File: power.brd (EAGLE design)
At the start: 136 x 136 mm, 38 parts, among them CN1 21700, CN2 21700, CN3 21700, CN4 21700, CN5 15PIN 0.5MM, Q1 IRLML6244, Q2 IRLML6244, U1 MAX17320G20+

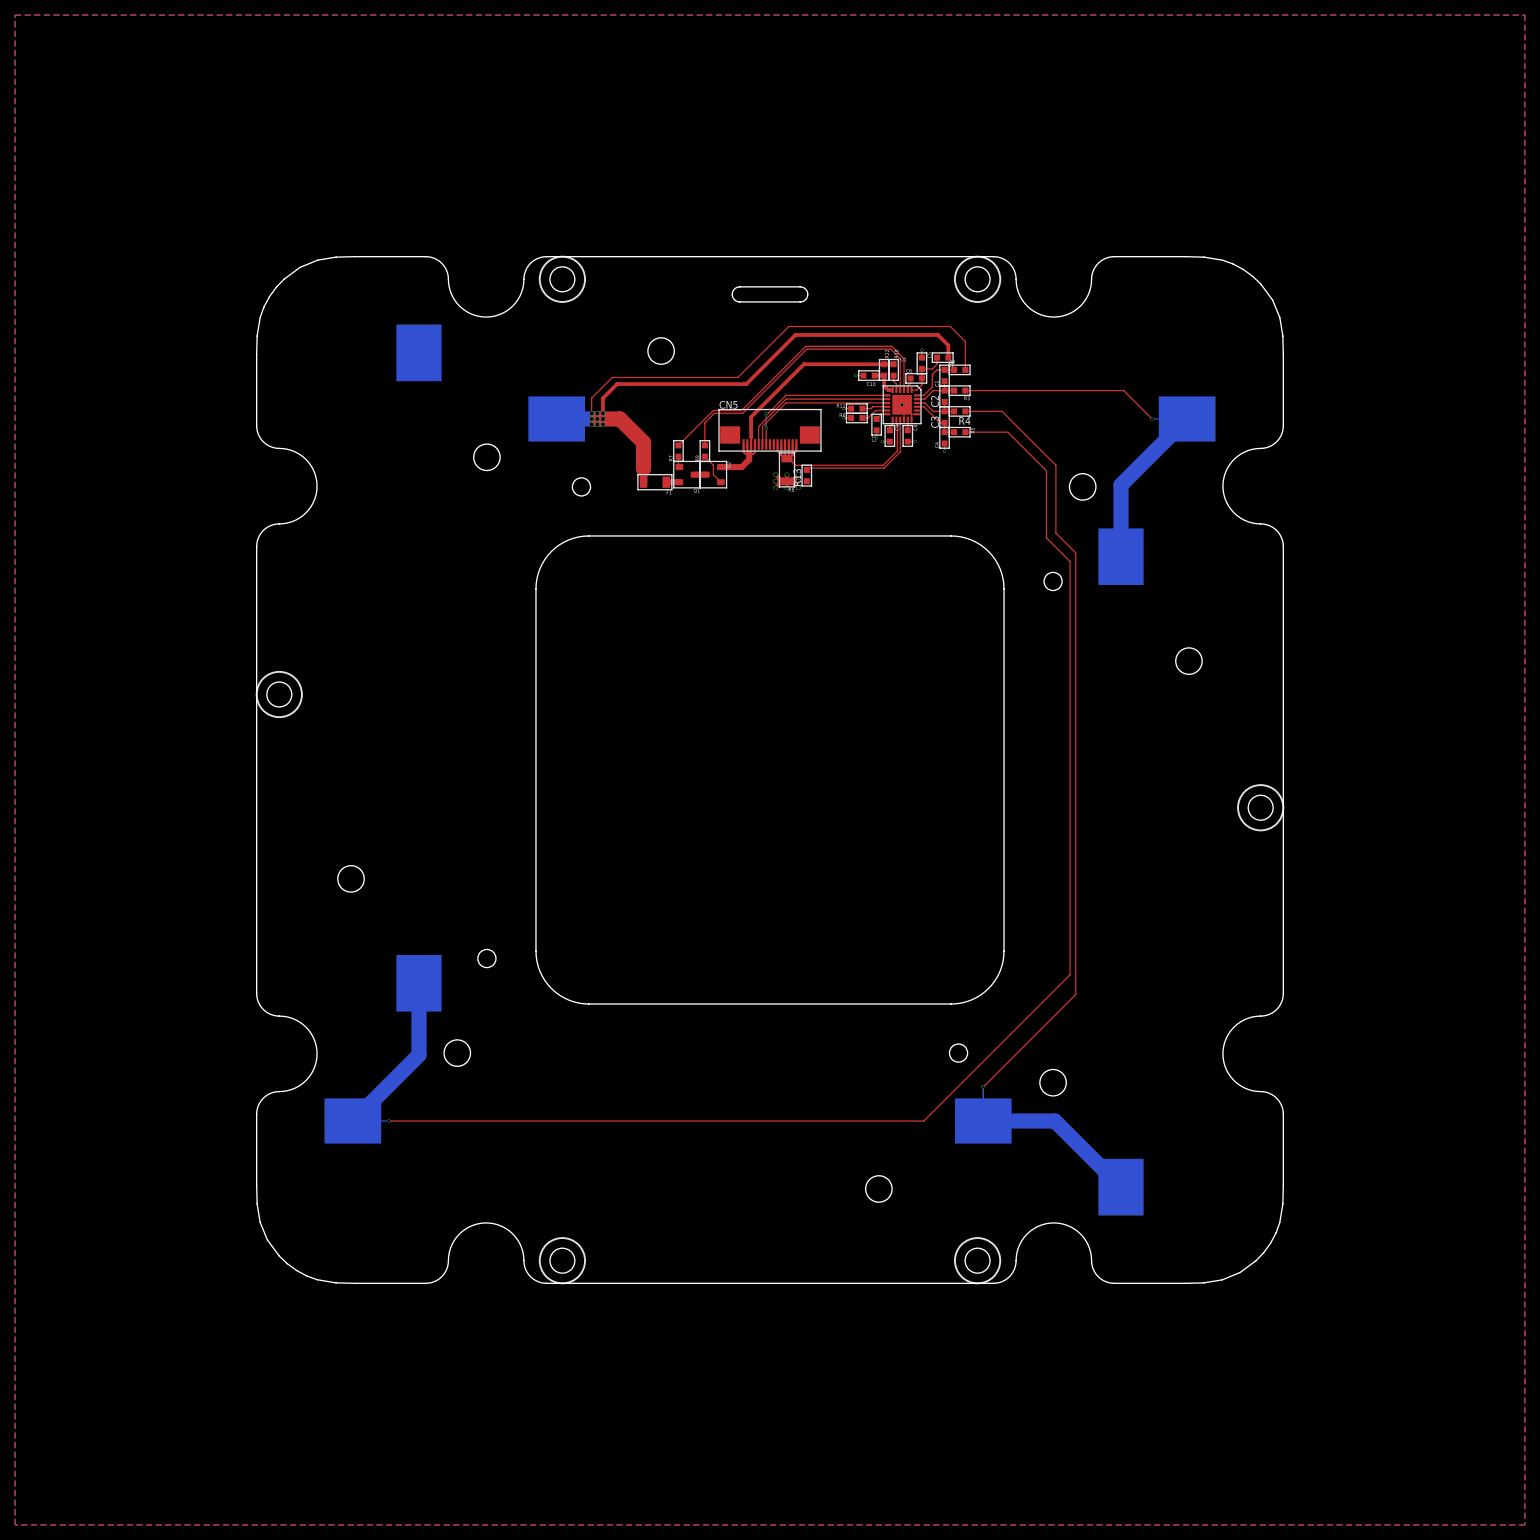
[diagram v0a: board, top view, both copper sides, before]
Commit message: New format working on
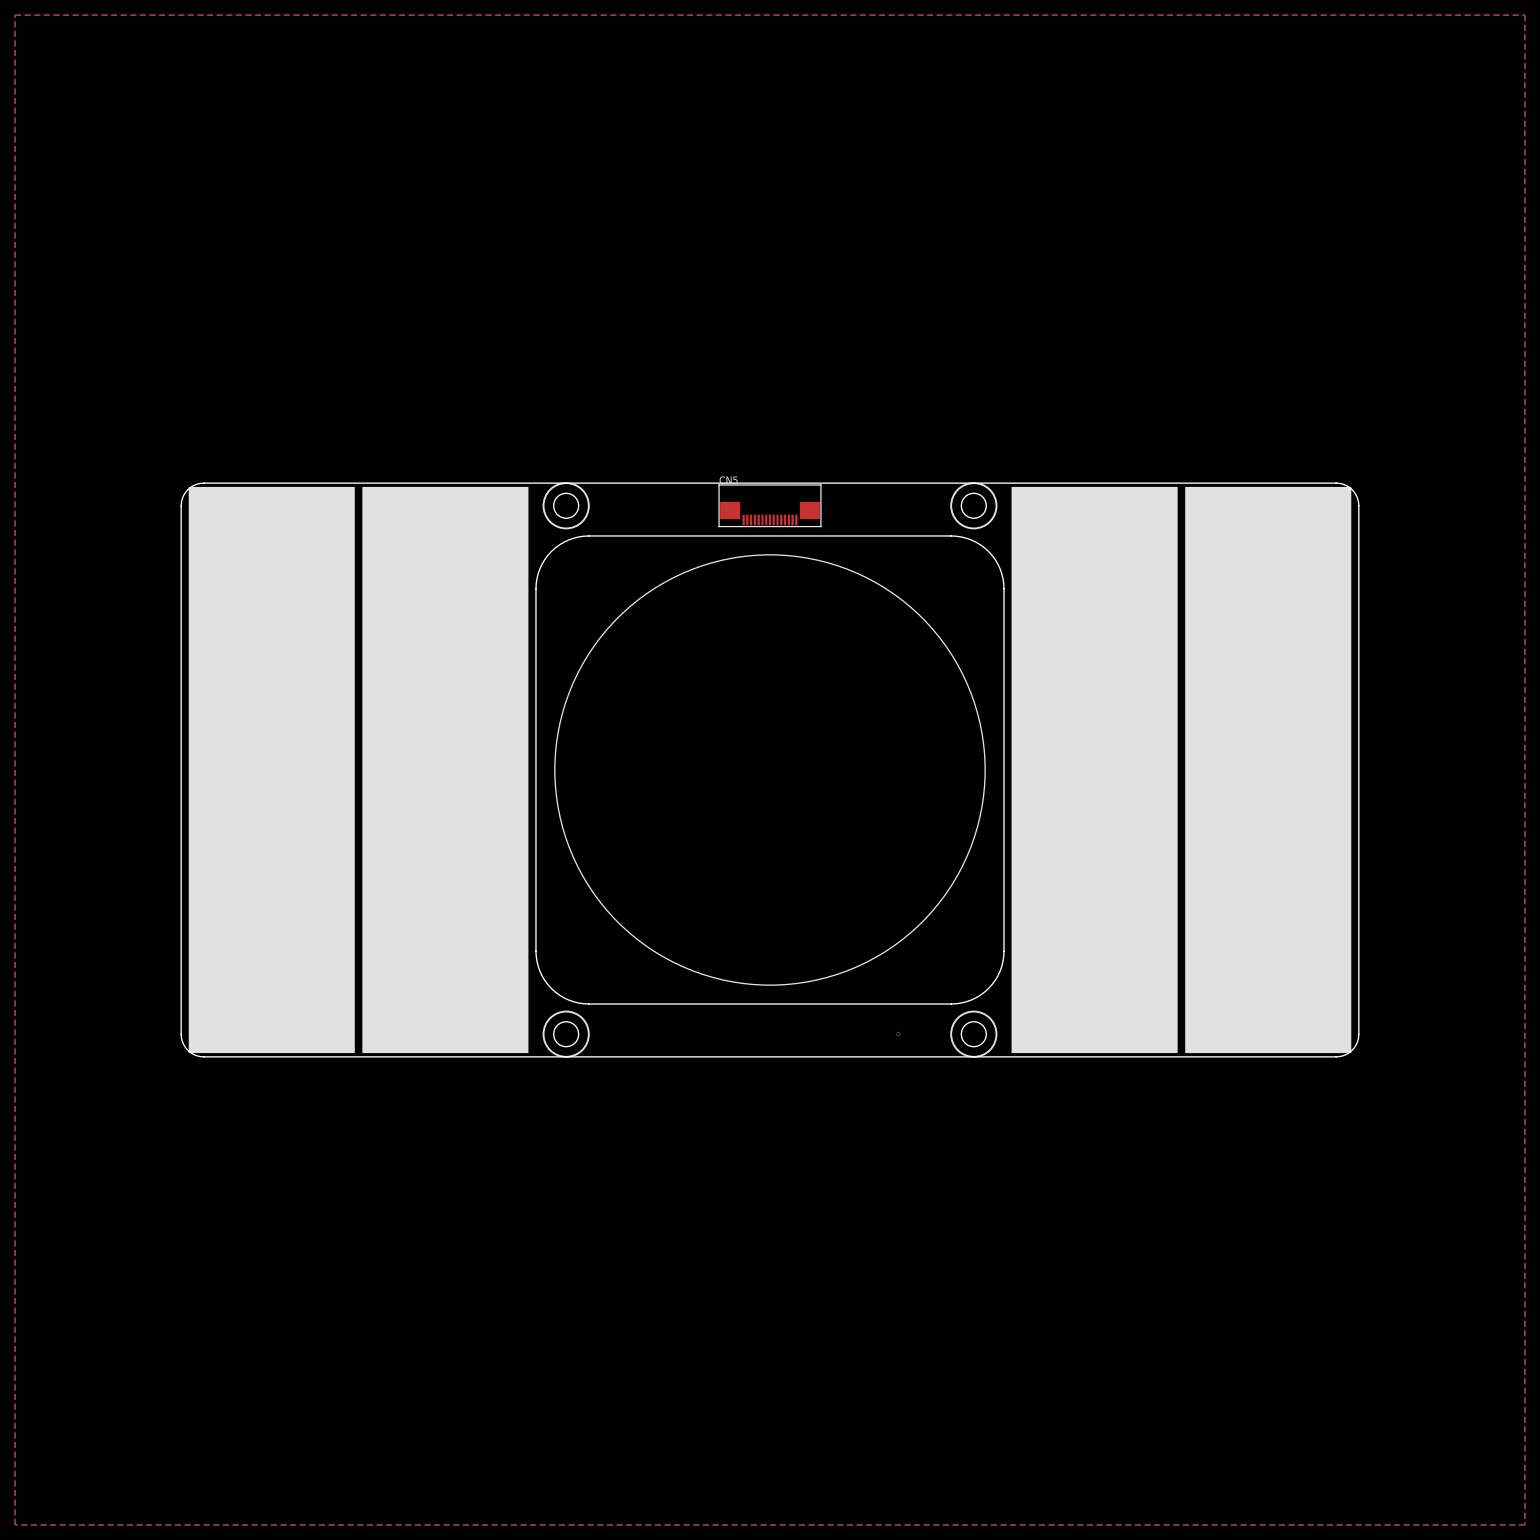
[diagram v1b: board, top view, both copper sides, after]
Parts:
- removed CN1, CN2, CN3, CN4: 21700, CONNECTORs:1122
- removed MECH1, MECH2, MECH4, MECH5: 6mm x 3mm, MISC:MOUNTHOLE_6X3
- added MECH7, MECH8: 6mm x 3mm, MISC:MOUNTHOLE_6X3
- moved MECH6 55.2 mm to (27.0, 35.0)
- moved MECH3 45.5 mm to (-27.0, 35.0)
- moved C1 38.8 mm to (48.2, 22.6)
- moved C10 38.8 mm to (38.2, 22.6)
- moved C2 38.8 mm to (48.2, 19.9)
- moved C3 38.8 mm to (48.2, 17.1)
- moved C4 38.8 mm to (48.2, 14.4)
- moved C5 38.8 mm to (45.2, 24.2)
- moved C6 38.8 mm to (44.5, 22.2)
- moved C7 38.8 mm to (39.2, 16.1)
- moved C8 38.8 mm to (43.4, 14.6)
- moved C9 38.8 mm to (41.0, 14.6)
- moved R1 38.8 mm to (48.0, 25.0)
- moved R10 38.8 mm to (41.5, 23.4)
- moved R11 38.8 mm to (36.6, 18.2)
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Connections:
- net N$36: no longer CN1.+
- net N$4: no longer CN1.-, CN2.+
- net N$5: no longer CN2.-, CN3.+
- net PACK_MID: no longer CN3.-, CN4.+
- net PGND: no longer CN4.-
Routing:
- net PACK_MID: track 205.8 -> 0.00 mm, vias 1 -> 0
- net N$36: track 141.5 -> 0.00 mm, vias 9 -> 0
- net N$5: track 129.9 -> 0.00 mm, vias 1 -> 0
- net N$4: track 52.8 -> 0.00 mm, vias 1 -> 0
- net N$59: track 40.2 -> 0.00 mm
- net N$56: track 37.6 -> 0.00 mm
- net PWR_VPACK: track 36.7 -> 0.00 mm
- net GND: track 31.5 -> 0.00 mm
- net PGND: track 23.4 -> 0.00 mm, vias 17 -> 1
- net BMS_NALERT: track 21.2 -> 0.00 mm, vias 2 -> 0
- net BMS_I2C_SCL: track 20.9 -> 0.00 mm
- net BMS_I2C_SDA: track 20.2 -> 0.00 mm
- net N$6: track 17.7 -> 0.00 mm
- net N$39: track 7.27 -> 0.00 mm
- net N$1: track 7.05 -> 0.00 mm
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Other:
- board size 136 x 136 mm -> 156 x 76 mm

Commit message: Progress
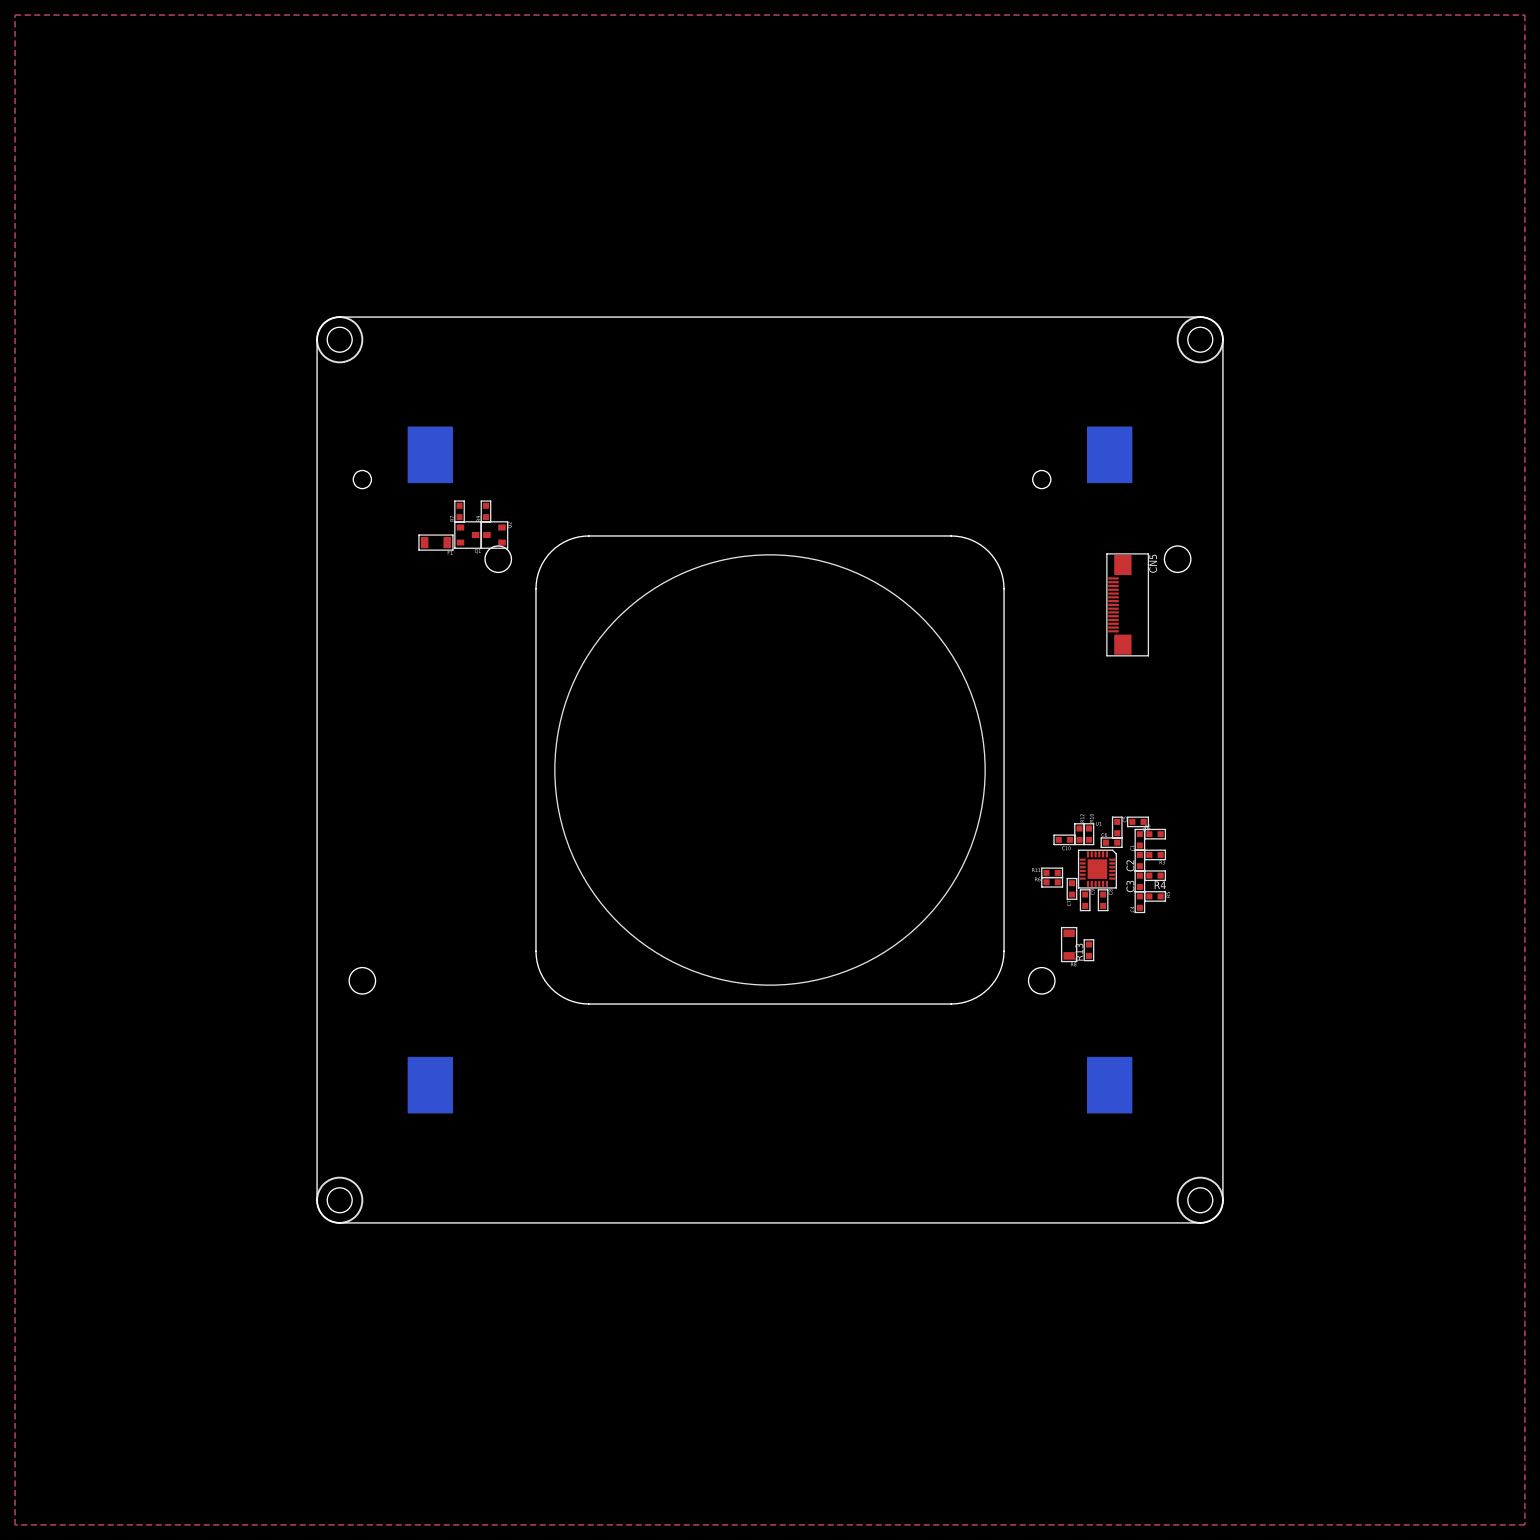
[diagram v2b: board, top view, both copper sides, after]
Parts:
- added CN1, CN2: 21700, CONNECTORs:1122
- moved R13 57.0 mm to (42.2, -23.9)
- moved R8 57.0 mm to (39.6, -23.1)
- moved CN5 49.2 mm to (47.4, 21.9), turned to 270 degrees
- moved MECH3 37.2 mm to (-57.0, 57.0)
- moved MECH6 37.2 mm to (57.0, 57.0)
- moved MECH7 37.2 mm to (-57.0, -57.0)
- moved MECH8 37.2 mm to (57.0, -57.0)
- moved C1 31.9 mm to (49.0, -9.25)
- moved C10 31.9 mm to (39.0, -9.25)
- moved C2 31.9 mm to (49.0, -12.0)
- moved C3 31.9 mm to (49.0, -14.8)
- moved C4 31.9 mm to (49.0, -17.5)
- moved C5 31.9 mm to (46.0, -7.62)
- moved C6 31.9 mm to (45.2, -9.62)
- moved C7 31.9 mm to (40.0, -15.8)
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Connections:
- net N$5: now also CN2.+
- net PACK_MID: now also CN1.+, CN2.-
- net PGND: now also CN1.-
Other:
- board size 156 x 76 mm -> 120 x 120 mm
